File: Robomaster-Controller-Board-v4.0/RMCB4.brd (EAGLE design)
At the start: 160 x 100 mm, 97 parts, among them J1 XT30PW-M, Q1 3.1A/30V/105mΩ, SW1 EG1319, U2 AP2112-3.3, X4 32.768, Y2 12mhz

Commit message: Thursday Meeting changes to the brd, waiting for final submit
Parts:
- removed AUX_GPIO1: S2B-PH-SM4_TB, KevinMade:S2B-PH-SM4_TB
- removed C27: 22pF, microbuilder:RESPACK_4X0603
- removed C28: 47nF, microbuilder:RESPACK_4X0603
- removed D+1, D-1: TPB1,27, testpad:B1,27
- removed PC1_PLED: RED, microbuilder:CHIPLED_0805_NOOUTLINE
- removed R15, R16: 10K, microbuilder:RESPACK_4X0603_NO
- removed R3: 10K, microbuilder:RESPACK_4X0603
- added C15: 47nF, microbuilder:0603-NO
- added C17, C24, C25: 22pF, microbuilder:0603-NO
- added C26: 100nF, microbuilder:0603-NO
- added PC1: (no value), adafruit:CHIPLED_0603
- added RELAY4: S2B-PH-SM4_TB, KevinMade:S2B-PH-SM4_TB
- added RN1, RN2: 10k, SparkFun-Resistors:0805-ARV
- added SSR4: G3VM-61VY2, SamacSys_Parts:SOP254P700X230-4N
- added U$31, U$32, U$35, U$37: MOUNTINGHOLE2.5, microbuilder:MOUNTINGHOLE_2.5_PLATED
- C10: device microbuilder:0805-NO -> microbuilder:0603-NO
- C18, C22: device microbuilder:0603-NO -> rcl:C0603
- C19, C20, C21: device microbuilder:0805-NO -> rcl:C0603
- C23: device microbuilder:RESPACK_4X0603 -> microbuilder:0603-NO
- C7, C9: value 10µF -> 10uF; device microbuilder:0805-NO -> microbuilder:0603-NO
- R1, R2: device microbuilder:RESPACK_4X0603 -> rcl:R0603
- R10, R14, R9: device microbuilder:0805-NO -> rcl:R0603
- R11, R19: device microbuilder:RESPACK_4X0603_NO -> rcl:R0603
- R12, R13, R17, R18, R20, R27: device microbuilder:0603-NO -> rcl:R0603
- moved J1 313.9 mm to (88.6, 7.62), turned to 270 degrees
- moved C8 313.7 mm to (30.7, 22.1), turned to 180 degrees
- moved C14 313.2 mm to (34.5, 19.6)
- moved CONN1 312.7 mm to (35.1, 44.2), turned to 180 degrees
- moved C11 310.2 mm to (34.5, 17.4)
- moved C12 307.2 mm to (30.7, 24.6), turned to 180 degrees
- moved Q1 305.9 mm to (30.0, 7.49)
- moved C16 305.5 mm to (30.7, 19.6), turned to 180 degrees
- moved SWITCH 305.4 mm to (21.1, 49.5), flipped to the bottom, turned to 180 degrees
- moved C13 303.6 mm to (34.5, 22.1)
- moved U2 303.0 mm to (34.5, 12.2)
- moved R20 301.0 mm to (33.5, 6.48), turned to 180 degrees
- moved C10 300.2 mm to (34.5, 24.6)
- moved C9 297.5 mm to (34.5, 15.4)
- moved C7 297.2 mm to (33.5, 8.38)
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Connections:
- removed net BACKUP1: AUX_GPIO1.1, U$40.24
- new net D14: SSR4.1, U$40.24
- new net RELAY4: RELAY4.1, SSR4.3
- net 24V: now also SSR4.4
- net 3.3V: now also C26.1, RN1.5, RN1.6, RN1.7, RN1.8, RN2.6, RN2.7; no longer R1.4, R15.5, R16.6, R2.4, R3.2, R3.4
- net D+: no longer D+1.TP
- net D-: no longer D-1.TP
- net FLASH_CS: now also R1.1; no longer R15.4
- net FLASH_MOSI: now also R11.1; no longer R11.4
- net GND: now also C15.2, C17.2, C23.2, C24.2, C25.2, C26.2, PC1.C, R11.2, R19.1, RELAY4.2, SSR4.2; no longer AUX_GPIO1.2, C23.5, C23.6, C23.7, C27.7, C28.8, PC1_PLED.C, R11.5, R19.3
- net I2C-1_CL: now also RN2.2; no longer R3.7
- net I2C-1_DA: now also RN2.3; no longer R3.5
- net I2C-2_CL: now also RN1.1; no longer R1.7
- net I2C-2_DA: now also RN1.2; no longer R1.5
- net I2C-3_CL: now also RN1.3; no longer R2.7
- net I2C-3_DA: now also RN1.4; no longer R2.5
- net N$10: now also C23.1; no longer C23.3
- net N$11: now also C24.1; no longer C23.2
- net N$12: now also C17.1; no longer C27.2
- net N$13: now also PC1.A; no longer PC1_PLED.A
- net N$22: now also C15.1; no longer C28.1
- net N$9: now also C25.1; no longer C23.4
- net SDIO_D3: now also R2.1; no longer R16.3
- net VBUS: now also R19.2; no longer R19.6
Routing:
- net 3.3V: track 45.9 -> 63.4 mm
- net EN: track 0.00 -> 8.95 mm, vias 0 -> 2
- net N$11: track 0.00 -> 6.85 mm
- net N$12: track 0.00 -> 6.82 mm
- net VHI: track 0.00 -> 6.60 mm
- net N$10: track 0.00 -> 6.39 mm
- net MODE_LED: track 6.20 -> 0.00 mm
- net N$9: track 0.00 -> 5.61 mm
- net CONNECTED_LED: track 5.66 -> 0.11 mm
- net N$22: track 0.00 -> 5.36 mm
- net VBUS: track 0.00 -> 3.31 mm
- net CAN_P: track 0.00 -> 2.35 mm
- net CAN_N: track 0.00 -> 2.35 mm
- net VCAP2: track 0.00 -> 2.19 mm, vias 0 -> 1
- net N$32: track 0.00 -> 1.88 mm
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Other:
- board size 160 x 100 mm -> 97.8 x 50.5 mm

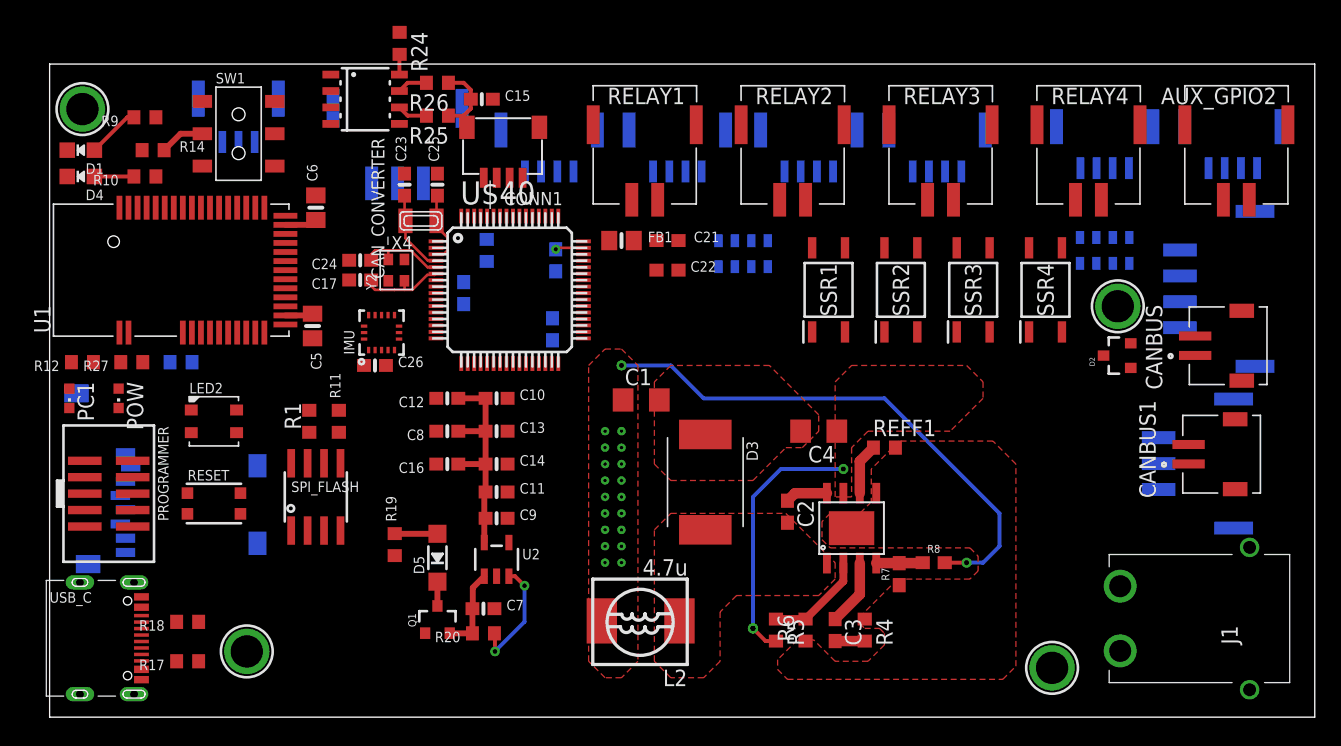
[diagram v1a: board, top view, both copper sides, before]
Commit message: final -kevin
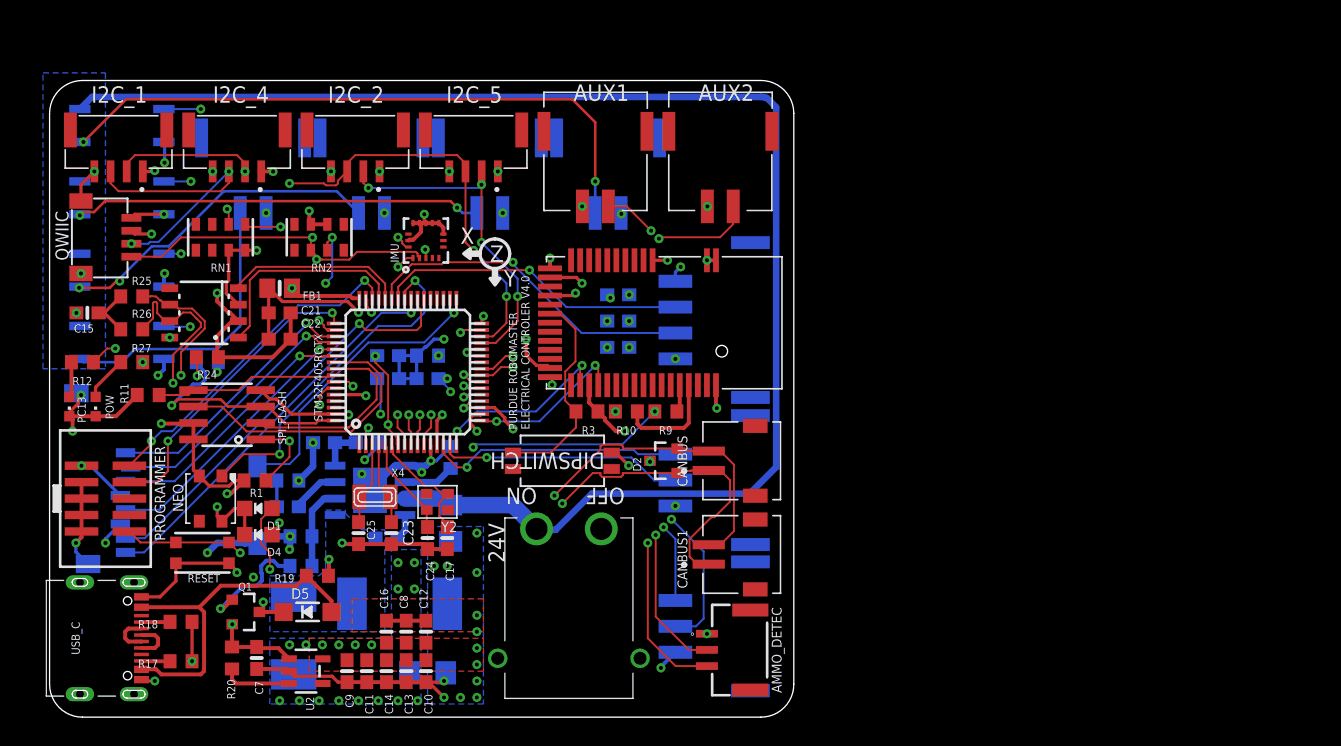
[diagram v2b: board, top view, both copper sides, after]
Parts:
- removed AUX_GPIO2: S2B-PH-SM4_TB, KevinMade:S2B-PH-SM4_TB
- removed CONN1: STEMMA_I2C_QT, microbuilder:JST_SH4
- removed I2C_3, I2C_6: SM04B-GHS-TB(LF)(SN)-, SM04B-GHS-TB_LF__SN_-:JST_SM04B-GHS-TB(LF)(SN)-
- removed J1: XT30PW-M, SamacSys_Parts:XT30PWM
- removed LED2: WS2812B3535, microbuilder:LED3535
- removed PC1: (no value), adafruit:CHIPLED_0603
- removed R14: 2K, rcl:R0603
- removed SW1: EG1319, microbuilder:EG1390
- removed U$31, U$32, U$35, U$37: MOUNTINGHOLE2.5, microbuilder:MOUNTINGHOLE_2.5_PLATED
- removed U$40: STM32F405R, adafruit_micro:TQFP64
- removed U$6: BM03-GHS_TBT, SamacSys_Parts:BM03-GHS-TBT
- added 24V: XT30PW-M, SamacSys_Parts:XT30PWM
- added AMMO_DETEC: BM03-GHS_TBT, SamacSys_Parts:BM03-GHS-TBT
- added AUX1, AUX2: S2B-PH-SM4_TB, KevinMade:S2B-PH-SM4_TB
- added DIPSWITCH: 1571983-3, Switches:SWSO4_300X100P50B
- added NEO: WS2812B3535, microbuilder:LED3535
- added PC13: (no value), adafruit:CHIPLED_0603
- added QWIIC: STEMMA_I2C_QT, microbuilder:JST_SH4
- added R3: 2K, rcl:R0603
- added STM32F405RGTX: STM32F405R, adafruit_micro:TQFP64
- C26: device microbuilder:0603-NO -> rcl:C0603
- C5, C6: device microbuilder:0805-NO -> rcl:C0603
- moved I2C_4 77.0 mm to (14.5, 44.5), flipped to the top
- moved I2C_1 76.2 mm to (5.33, 44.5), flipped to the top
- moved RELAY4 74.2 mm to (10.9, 47.2), flipped to the bottom
- moved SSR4 71.5 mm to (5.59, 29.0), flipped to the bottom, turned to 0 degrees
- moved SSR3 65.8 mm to (5.59, 34.5), flipped to the bottom, turned to 0 degrees
- moved RN2 60.7 mm to (20.8, 37.1), flipped to the top, turned to 0 degrees
- moved SSR2 60.6 mm to (5.59, 40.1), flipped to the bottom, turned to 0 degrees
- moved SSR1 56.1 mm to (5.59, 45.7), flipped to the bottom, turned to 0 degrees
- moved RELAY3 53.6 mm to (20.1, 47.2), flipped to the bottom
- moved SWITCH 51.1 mm to (56.6, 12.8), turned to 270 degrees
- moved R9 46.2 mm to (47.6, 23.6)
- moved R4 46.1 mm to (18.4, 18.3), flipped to the bottom, turned to 0 degrees
- moved R7 45.6 mm to (21.2, 21.2), flipped to the bottom, turned to 180 degrees
- moved R8 44.8 mm to (24.5, 21.2), flipped to the bottom, turned to 180 degrees
- moved C3 43.4 mm to (18.4, 16.3), flipped to the bottom, turned to 0 degrees
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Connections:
- removed net BACKUP2: AUX_GPIO2.1, U$40.25
- removed net D10: U$40.62
- removed net D8_NEOPIX: LED2.1, U$40.8
- removed net D9: U$40.61
- removed net I2C-3_CL: I2C_3.2, I2C_6.2, RN1.3, U$40.41
- removed net I2C-3_DA: I2C_3.3, I2C_6.3, RN1.4, U$40.40
- removed net MISO: U$40.35
- removed net MOSI: U$40.36
- removed net N$4: R14.2, SW1.P2
- removed net SCK: U$40.34
- new net GPIO_AUX1: AUX1.1, STM32F405RGTX.25
- new net GPIO_AUX2: AUX2.1, STM32F405RGTX.24
- new net NEOPIX: NEO.1, STM32F405RGTX.41
- new net PB13: STM32F405RGTX.34
- new net PB14: STM32F405RGTX.35
- new net PB15: STM32F405RGTX.36
- new net PB8: STM32F405RGTX.61
- new net PB9: STM32F405RGTX.62
- new net PC13: R12.1, STM32F405RGTX.2
- new net PC6: STM32F405RGTX.37
- new net PC7: STM32F405RGTX.38
- net !RESET: now also STM32F405RGTX.7; no longer U$40.7
- net 24V: now also 24V.2; no longer J1.2
- net 3.3V: now also DIPSWITCH.2, NEO.2, QWIIC.2, STM32F405RGTX.19, STM32F405RGTX.32, STM32F405RGTX.48, STM32F405RGTX.64; no longer CONN1.2, I2C_3.1, I2C_6.1, LED2.2, RN1.5, RN1.6, SW1.O2, U$40.19, U$40.32, U$40.42, U$40.43, U$40.48, U$40.64
- net AMMO1: now also AMMO_DETEC.1, STM32F405RGTX.20; no longer U$40.20, U$6.1
- net AMMO2: now also AMMO_DETEC.2, STM32F405RGTX.21; no longer U$40.21, U$6.2
- net BOARD_RX: now also STM32F405RGTX.15; no longer U$40.15
- net BOARD_TX: now also STM32F405RGTX.14; no longer U$40.14
- net BOOT0: now also STM32F405RGTX.60; no longer U$40.60
- net CANRX_N: now also STM32F405RGTX.44; no longer U$40.44
- net CANTX_P: now also STM32F405RGTX.45; no longer U$40.45
- net D11: now also STM32F405RGTX.11; no longer U$40.11
- net D12: now also STM32F405RGTX.10; no longer U$40.10
- net D13: now also STM32F405RGTX.9; no longer R12.1, U$40.9
- net D14: now also STM32F405RGTX.8; no longer U$40.24
- net FLASH_CS: now also STM32F405RGTX.50; no longer U$40.50
- net FLASH_MISO: now also STM32F405RGTX.56; no longer U$40.56
- net FLASH_MOSI: now also STM32F405RGTX.57; no longer U$40.57
- net FLASH_SCK: now also STM32F405RGTX.55; no longer U$40.55
- net GND: now also 24V.1, AMMO_DETEC.3, AUX1.2, AUX2.2, NEO.4, PC13.C, QWIIC.1, QWIIC.MT1, QWIIC.MT2, R3.1, STM32F405RGTX.12, STM32F405RGTX.18, STM32F405RGTX.28, STM32F405RGTX.63; no longer AUX_GPIO2.2, CONN1.1, CONN1.MT1, CONN1.MT2, I2C_3.4, I2C_6.4, J1.1, LED2.4, PC1.C, SW1.S2, U$40.12, U$40.18, U$40.28, U$40.63, U$6.3
- net I2C-1_CL: now also QWIIC.4, STM32F405RGTX.58; no longer CONN1.4, U$40.58
- net I2C-1_DA: now also QWIIC.3, STM32F405RGTX.59; no longer CONN1.3, U$40.59
- net I2C-2_CL: now also STM32F405RGTX.29; no longer U$40.29
- net I2C-2_DA: now also STM32F405RGTX.30; no longer U$40.30
- net MODE_3V: now also DIPSWITCH.3, R3.2; no longer R14.1
- net N$10: now also STM32F405RGTX.4; no longer U$40.4
- net N$11: now also STM32F405RGTX.5; no longer U$40.5
- net N$12: now also STM32F405RGTX.6; no longer U$40.6
- net N$13: now also PC13.A; no longer PC1.A
- net N$20: now also STM32F405RGTX.13; no longer U$40.13
- net N$9: now also STM32F405RGTX.3; no longer U$40.3
- net PB0: now also STM32F405RGTX.26; no longer U$40.26
- net PB1: now also STM32F405RGTX.27; no longer U$40.27
- net RX_BT: now also STM32F405RGTX.17; no longer U$40.17
- net SDIO_CLK: now also STM32F405RGTX.53; no longer U$40.38
- net SDIO_CMD: now also STM32F405RGTX.54; no longer U$40.37
- net SDIO_D0: now also STM32F405RGTX.39; no longer U$40.39
- net SDIO_D1: now also STM32F405RGTX.40; no longer U$40.2
- net SDIO_D2: now also STM32F405RGTX.51; no longer U$40.51
- net SDIO_D3: now also STM32F405RGTX.52; no longer U$40.52
- net SD_DETECT: now also STM32F405RGTX.33; no longer U$40.33
- net SHIELD: no longer I2C_3.SH1, I2C_3.SH2, I2C_6.SH1, I2C_6.SH2
- net SWCLK: now also STM32F405RGTX.49; no longer U$40.49
- net SWDIO: now also STM32F405RGTX.46; no longer U$40.46
- net SWITCH1: now also STM32F405RGTX.22; no longer U$40.22
- net SWITCH2: now also STM32F405RGTX.23; no longer U$40.23
- net TX_BT: now also STM32F405RGTX.16; no longer U$40.16
- net VCAP1: now also STM32F405RGTX.31; no longer U$40.31
- net VCAP2: now also STM32F405RGTX.47; no longer U$40.47
- net VISION_RX: now also STM32F405RGTX.43; no longer U$40.54
- net VISION_TX: now also STM32F405RGTX.42; no longer U$40.53
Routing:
- net GND: track 0.00 -> 151.8 mm, vias 0 -> 67
- net 24V: track 20.2 -> 150.1 mm, vias 3 -> 1
- net CAN_P: track 2.35 -> 71.1 mm, vias 0 -> 2
- net CAN_N: track 2.35 -> 67.1 mm, vias 0 -> 2
- net I2C-1_DA: track 0.00 -> 60.1 mm, vias 0 -> 6
- net I2C-1_CL: track 0.00 -> 55.9 mm, vias 0 -> 4
- net RELAY1: track 0.00 -> 48.9 mm, vias 0 -> 2
- net D11: track 0.00 -> 41.9 mm, vias 0 -> 2
- net I2C-2_DA: track 0.00 -> 38.3 mm, vias 0 -> 4
- net I2C-2_CL: track 0.00 -> 37.4 mm, vias 0 -> 5
- net N$6: track 3.05 -> 39.5 mm, vias 0 -> 3
- net N$5: track 4.11 -> 40.1 mm, vias 0 -> 3
- net D12: track 0.00 -> 35.3 mm, vias 0 -> 2
- net SWITCH2: track 0.00 -> 33.4 mm, vias 0 -> 2
- net AMMO1: track 0.00 -> 33.0 mm, vias 0 -> 2
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- added copper zone on layer 16, net 24V
- added copper zone on layer 15, net 3.3V
- added copper zone on layer 16, net 3.3V
- added copper zone on layer 16, net GND
- added copper zone on layer 2, net GND
- added copper zone on layer 16, net SW1
- removed copper zone on layer 1, net 24V
- removed copper zone on layer 1, net SW1
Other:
- board size 97.8 x 50.5 mm -> 57.5 x 49.2 mm
- board text added: "PURDUE ROBOMASTER ELECTRICAL CONTROLER V4.0"
- board text added: "SCH: HENRY SILVA / ALBERT SUN SIYU WU / MATTHEW AGNEW BRD: CHENGMING ZHANG"
- board text added: "X"
- board text added: "Y"
- board text added: "Z"
